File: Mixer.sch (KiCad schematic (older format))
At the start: 91 parts, among them J100 Conn_01x01, J101 Conn_01x01, J126 Conn_Coaxial, J127 Conn_Coaxial, J128 Conn_01x01, J129 Conn_01x01, J130 Conn_01x01, J131 Conn_01x01, J92 Conn_Coaxial, J93 Conn_Coaxial, J94 Conn_Coaxial, J95 Conn_Coaxial, J96 Conn_Coaxial, J97 Conn_Coaxial, J98 Conn_01x01, J99 Conn_01x01, Q16 2SC3356, Q17 2SC3356, Q18 2SC3356, Q19 2SC3356, Q20 2SC3356, Q21 2SC3356, Q22 2SC3356, Q23 2SC3356, Q26 2SC3356, Q27 2SC3356, Q28 2SC3356

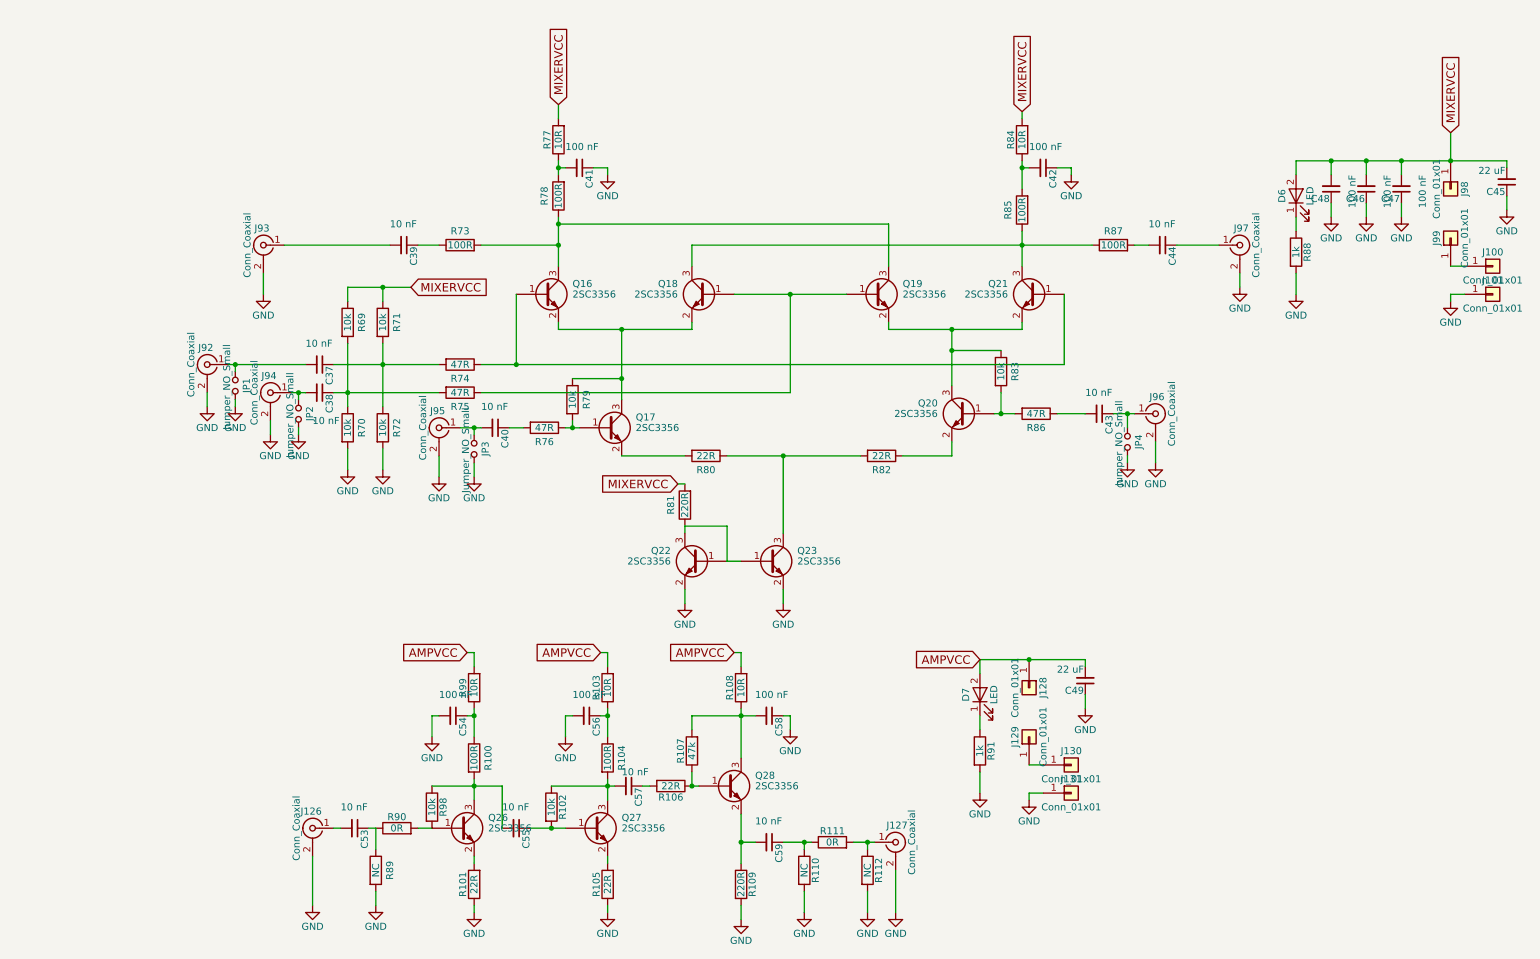
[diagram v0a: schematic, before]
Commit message: Submitted to JLCPCB 2020-07-12
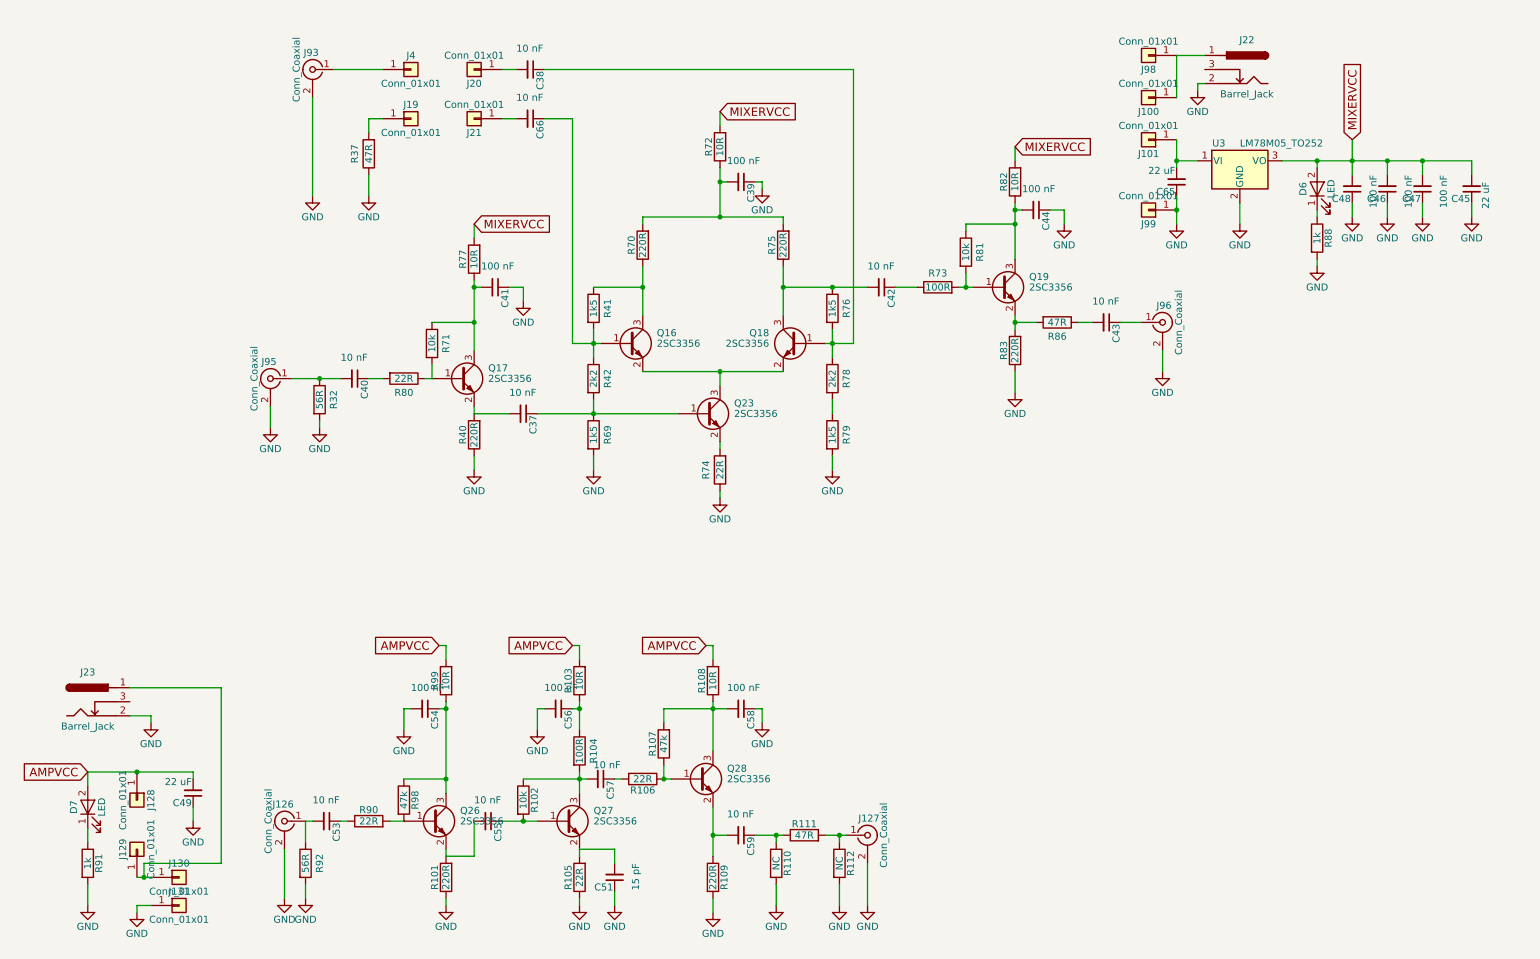
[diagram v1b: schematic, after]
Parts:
- removed J92, J94, J97: Conn_Coaxial, RFUtilityKnife:Amphenol_RF_SMA_132289, symbol Conn_Coaxial
- removed JP1, JP2, JP3, JP4: Jumper_NO_Small, Pin_Headers:Pin_Header_Straight_1x02_Pitch2.54mm, symbol Jumper_NO_Small
- removed Q20, Q21, Q22: 2SC3356, TO_SOT_Packages_SMD:SOT-23, symbol MMBT3904
- removed R100, R85, R87: 100R, Resistors_SMD:R_0805_HandSoldering, symbol R
- removed R84: 10R, Resistors_SMD:R_0805_HandSoldering, symbol R
- removed R89: NC, Resistors_SMD:R_0805_HandSoldering, symbol R
- added C51: 15 pF, Capacitors_SMD:C_0805_HandSoldering, symbol C_Small
- added C65: 22 uF, Capacitors_SMD:C_0805_HandSoldering, symbol C_Small
- added C66: 10 nF, Capacitors_SMD:C_0805_HandSoldering, symbol C_Small
- added J19, J20, J21, J4: Conn_01x01, RFUtilityKnife:PadHole, symbol Conn_01x01
- added J22, J23: Barrel_Jack, Connectors:BARREL_JACK, symbol Barrel_Jack
- added R32, R92: 56R, Resistors_SMD:R_0805_HandSoldering, symbol R
- added R37: 47R, Resistors_SMD:R_0805_HandSoldering, symbol R
- added R40: 220R, Resistors_SMD:R_0805_HandSoldering, symbol R
- added R41: 1k5, Resistors_SMD:R_0805_HandSoldering, symbol R
- added R42: 2k2, Resistors_SMD:R_0805_HandSoldering, symbol R
- added U3: LM78M05_TO252, TO_SOT_Packages_SMD:TO-252-3_TabPin2, symbol LM78M05_TO252
- C39, C44: value 10 nF -> 100 nF; LCSC C1710 -> C49678
- C42: value 100 nF -> 10 nF; LCSC C49678 -> C1710
- R101: value 22R -> 220R; LCSC C17561 -> C17557
- R111: value 0R -> 47R; LCSC C17477 -> C17714
- R69, R79: value 10k -> 1k5; LCSC C17414 -> C4310
- R70, R83: value 10k -> 220R; LCSC C17414 -> C17557
- R72: value 10k -> 10R; LCSC C17414 -> C17415
- R74: value 47R -> 22R; LCSC C17714 -> C17561
- R75: value 47R -> 220R; LCSC C17714 -> C17557
- R76: value 47R -> 1k5; LCSC C17714 -> C4310
- R78: value 100R -> 2k2; LCSC C17408 -> C17520
- R81: value 220R -> 10k; LCSC C17557 -> C17414
- R82: value 22R -> 10R; LCSC C17561 -> C17415
- R90: value 0R -> 22R; LCSC C17477 -> C17561
- R98: value 10k -> 47k; LCSC C17414 -> C17713
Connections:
- net GND: now also C39.1, C44.1, J99.1 (Pin_1), R69.2, R74.1, R79.2, R83.1, C51.1, C65.1, J22.2, J23.2, R32.2, R37.1, R40.1, R92.2, U3.2 (GND); no longer C42.1, J101.1 (Pin_1), Q23.2 (E), R70.2, R72.2
- net MIXERVCC: now also R72.2, R82.2, U3.3 (VO); no longer J98.1 (Pin_1), R69.1, R71.1, R81.2
- net at J100.1 (Pin_1): now also J98.1 (Pin_1), J22.1; no longer J99.1 (Pin_1)
- net at R80.2: now also C40.1; no longer Q17.2 (E)
- net at R82.1: now also C44.2, Q19.3 (C), R81.1
- net at C41.2, R77.1: now also Q17.3 (C), R71.1; no longer R78.2
- net at Q16.1 (B): now also C66.1, R41.2, R42.1; no longer R74.1
- net at Q16.2 (E), Q18.2 (E): now also Q23.3 (C); no longer Q17.3 (C), R79.1
- net at Q18.3 (C): now also C42.2, R75.1, R76.1
- net at Q19.2 (E): now also R83.2, R86.2; no longer R83.1
- net at C37.2: now also Q17.2 (E), R40.2
- net at C38.2: now also J20.1 (Pin_1)
- net at C40.2, J95.1 (In): now also R32.1
- net at R76.2: now also C38.1, Q18.1 (B), R78.1; no longer C40.1
- net at R73.1: now also C42.1; no longer C39.1
- net at J93.1 (In): now also J4.1 (Pin_1); no longer C39.2
- net at Q23.1 (B): now also C37.1, R69.1, R42.2; no longer R81.1
- net at Q26.3 (C), R98.1: now also C54.1, R99.1; no longer C55.2
- net at Q27.2 (E), R105.2: now also C51.2
- net at C53.2, J126.1 (In): now also R92.1
- net at Q26.2 (E), R101.2: now also C55.2
- net at J129.1 (Pin_1), J130.1 (Pin_1): now also J23.1
- new net: C65.2, J101.1 (Pin_1), U3.1 (VI)
- new net: Q17.1 (B), R71.2, R80.1
- new net: Q16.3 (C), R41.1, R70.1
- new net: Q19.1 (B), R73.2, R81.2
- new net: Q23.2 (E), R74.2
- new net: C39.2, R70.2, R72.1, R75.2
- new net: R78.2, R79.1
- new net: C66.2, J21.1 (Pin_1)
- new net: J19.1 (Pin_1), R37.2
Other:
- moved on the sheet: C40, C41, C43, C45, C46, C47, C48, C49, C53, C54, C55, C56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
